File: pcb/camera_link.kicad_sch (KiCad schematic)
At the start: 12 parts, among them J1 RJ45_pyControl, J2 Screw_Terminal_01x08

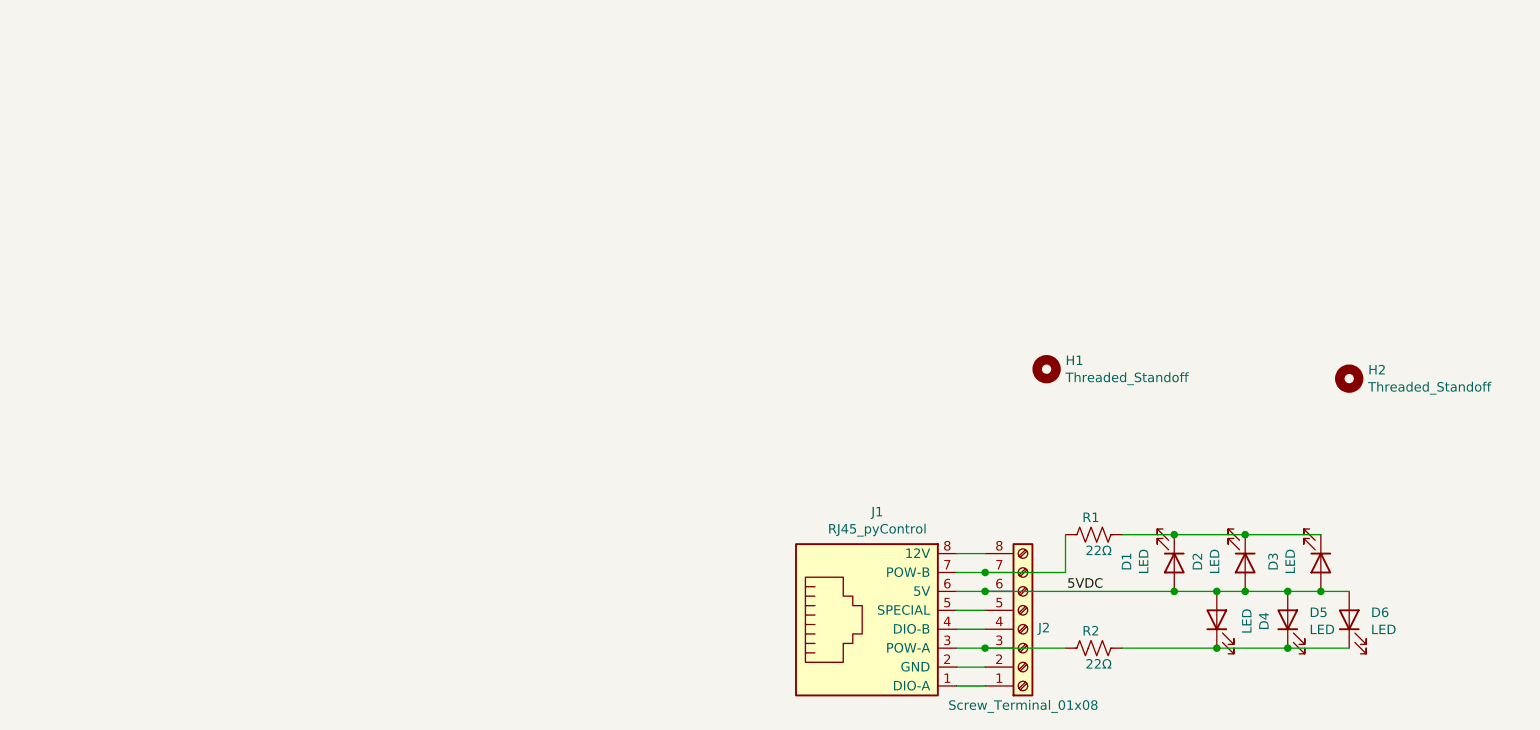
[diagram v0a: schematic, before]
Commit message: pcbv1.2
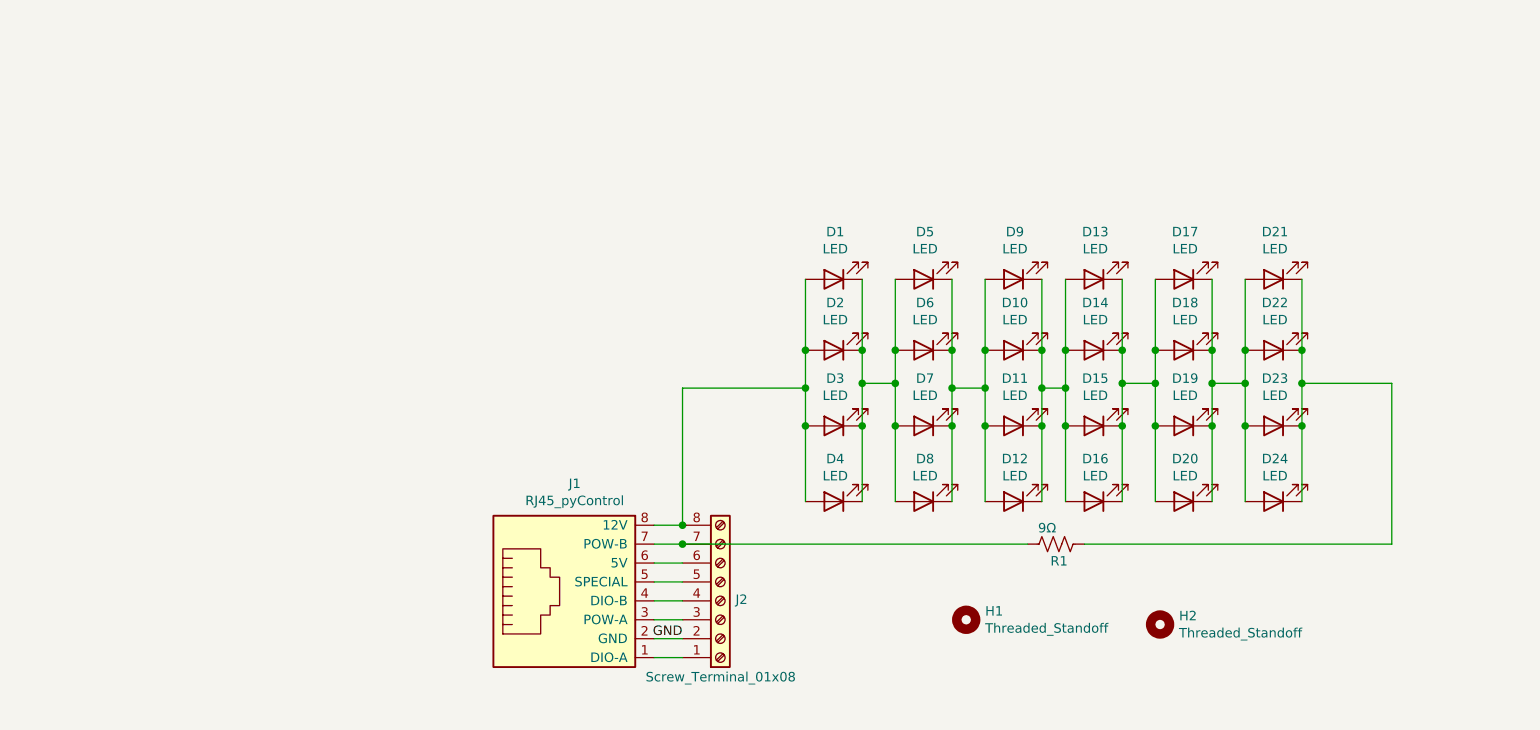
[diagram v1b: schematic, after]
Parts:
- removed R2: 22Ω, Resistor_THT:R_Axial_DIN0204_L3.6mm_D1.6mm_P7.62mm_Horizontal, symbol Device:R_US
- added D10, D11, D12, D13, D14, D15, D16, D17, D18, D19, D20, D21, D22, D23, D24, D7, D8, D9: LED, LED_SMD:LED_1206_3216Metric, symbol Device:LED
- J1: footprint asl_footprints:RJ45_THP_Vertical -> asl_footprints:RJ45_SMD
- R1: value 22Ω -> 9Ω; footprint Resistor_THT:R_Axial_DIN0204_L3.6mm_D1.6mm_P7.62mm_Horizontal -> Resistor_SMD:R_1206_3216Metric_Pad1.30x1.75mm_HandSolder
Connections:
- net GND: now reaches J1.2 (GND), J2.2 (Pin_2)
- net at J1.7 (POW-B), J2.7 (Pin_7): now also R1.2; no longer R1.1
- net at J1.8 (12V), J2.8 (Pin_8): now also D1.2 (A), D2.2 (A), D3.2 (A), D4.2 (A)
- net at D5.1 (K), D6.1 (K): now also D10.2 (A), D11.2 (A), D12.2 (A), D7.1 (K), D8.1 (K), D9.2 (A); no longer D4.1 (K)
- net at D1.1 (K), D2.1 (K), D3.1 (K): now also D4.1 (K), D5.2 (A), D6.2 (A), D7.2 (A), D8.2 (A); no longer R1.2
- removed net 5VDC: D1.2 (A), D2.2 (A), D3.2 (A), D4.2 (A), D5.2 (A), D6.2 (A), J1.6 (5V), J2.6 (Pin_6)
- new net: D17.1 (K), D18.1 (K), D19.1 (K), D20.1 (K), D21.2 (A), D22.2 (A), D23.2 (A), D24.2 (A)
- new net: D13.1 (K), D14.1 (K), D15.1 (K), D16.1 (K), D17.2 (A), D18.2 (A), D19.2 (A), D20.2 (A)
- new net: D10.1 (K), D11.1 (K), D12.1 (K), D13.2 (A), D14.2 (A), D15.2 (A), D16.2 (A), D9.1 (K)
- new net: J1.6 (5V), J2.6 (Pin_6)
- new net: D21.1 (K), D22.1 (K), D23.1 (K), D24.1 (K), R1.1
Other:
- moved on the sheet: D1, D2, D3, H1, H2, J1, J2, R1

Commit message: pcb v1.3
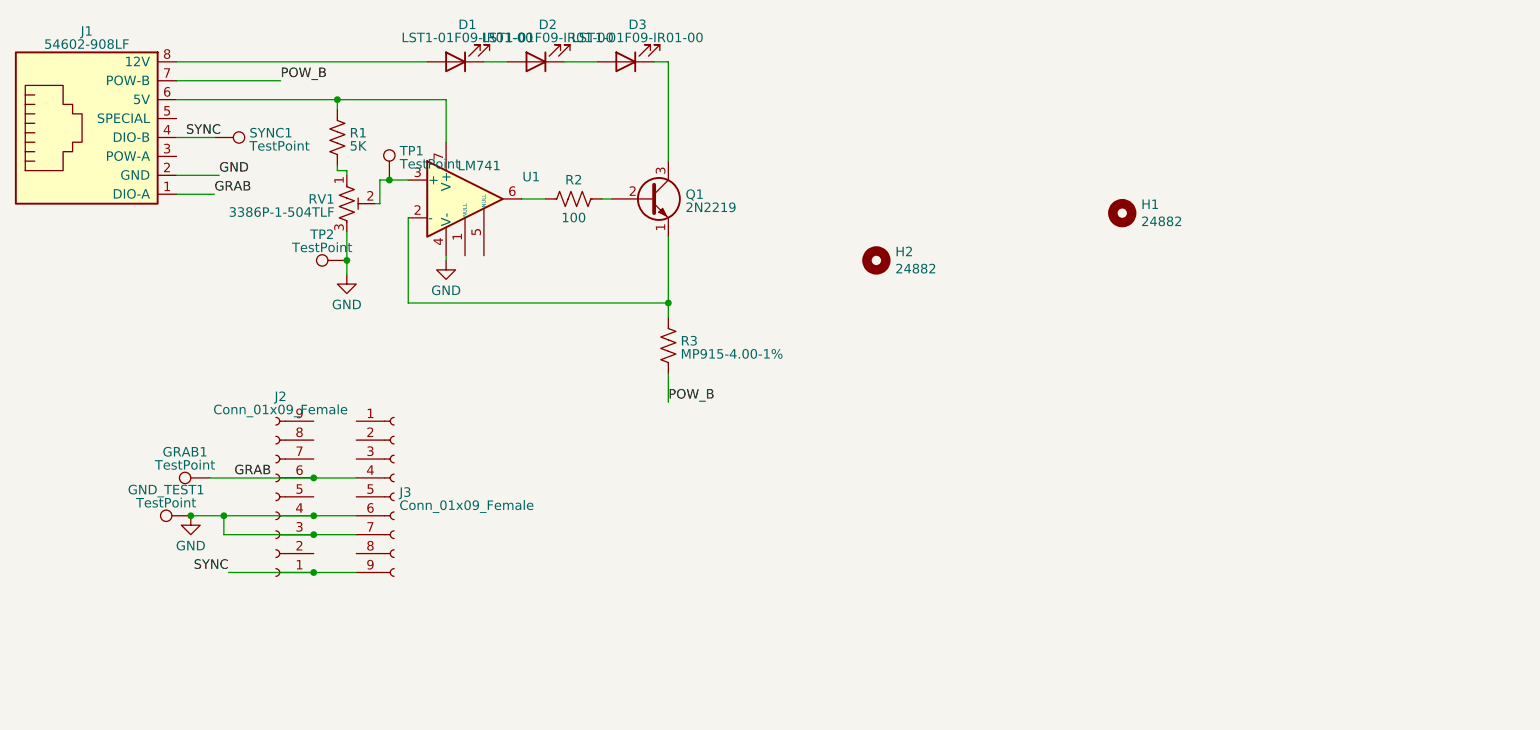
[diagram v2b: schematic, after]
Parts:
- removed D10, D11, D12, D13, D14, D15, D16, D17, D18, D19, D20, D21, D22, D23, D24, D4, D5, D6, D7, D8, D9: LED, LED_SMD:LED_1206_3216Metric, symbol Device:LED
- removed J2: Screw_Terminal_01x08, Connector_PinHeader_1.27mm:PinHeader_1x08_P1.27mm_Vertical, symbol Connector:Screw_Terminal_01x08
- added GND_TEST1, GRAB1, SYNC1, TP1, TP2: TestPoint, Connector_Pin:Pin_D1.0mm_L10.0mm, symbol Connector:TestPoint
- added J2, J3: Conn_01x09_Female, asl_footprints:JST_NSH_1x09_VERTICAL, symbol Connector:Conn_01x09_Female
- added Q1: 2N2219, Package_TO_SOT_SMD:SOT-23-6, symbol asl_symbols_new:NPN_transistor_ZXTC2045E6TA
- added R2: 100, Resistor_SMD:R_0805_2012Metric, symbol Device:R_US
- added R3: MP915-4.00-1%, asl_footprints:Resistor_power_MP900, symbol Device:R_US
- added RV1: 3386P-1-504TLF, Potentiometer_THT:Potentiometer_Bourns_3386P_Vertical, symbol Device:R_Potentiometer_Trim_US
- added U1: LM741, Package_DIP:DIP-8_W7.62mm, symbol Amplifier_Operational:LM741
- D1, D2, D3: value LED -> LST1-01F09-IR01-00; footprint LED_SMD:LED_1206_3216Metric -> asl_footprints:LED_starboard
- H1: renamed from H2; value Threaded_Standoff -> 24882; Sim_Device (none) -> SPICE; Sim_Params (none) -> type=H model="24882"
- H2: renamed from H1; value Threaded_Standoff -> 24882; Sim_Device (none) -> SPICE; Sim_Params (none) -> type=H model="24882"
- J1: value RJ45_pyControl -> 54602-908LF; footprint asl_footprints:RJ45_SMD -> asl_footprints:RJ45_THP
- R1: value 9Ω -> 5K; footprint Resistor_SMD:R_1206_3216Metric_Pad1.30x1.75mm_HandSolder -> Resistor_SMD:R_0805_2012Metric
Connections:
- net GND: now also GND_TEST1.1, J2.3 (Pin_3), J2.4 (Pin_4), J3.6 (Pin_6), J3.7 (Pin_7), RV1.3, TP2.1, U1.4 (V-)
- net GRAB: now reaches J1.1 (DIO-A)
- net GRAB: now also GRAB1.1, J2.6 (Pin_6), J3.4 (Pin_4)
- net SYNC: now reaches J1.4 (DIO-B)
- net SYNC: now also J2.1 (Pin_1), J3.9 (Pin_9), SYNC1.1
- net at J1.6 (5V): now also R1.1, U1.7 (V+)
- net at R1.2: now also RV1.1; no longer J1.7 (POW-B)
- net at D1.2 (A), J1.8 (12V): no longer D2.2 (A), D3.2 (A)
- new net: D2.1 (K), D3.2 (A)
- new net: D1.1 (K), D2.2 (A)
- new net: D3.1 (K), Q1.3 (C)
- new net: Q1.1 (E), R3.2, U1.2 (-)
- new net: RV1.2, TP1.1, U1.3 (+)
- new net: Q1.2 (B), R2.2
- new net: R2.1, U1.6
- new net POW_B: J1.7 (POW-B), R3.1
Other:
- moved on the sheet: H1, H2

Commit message: pcb v1.5
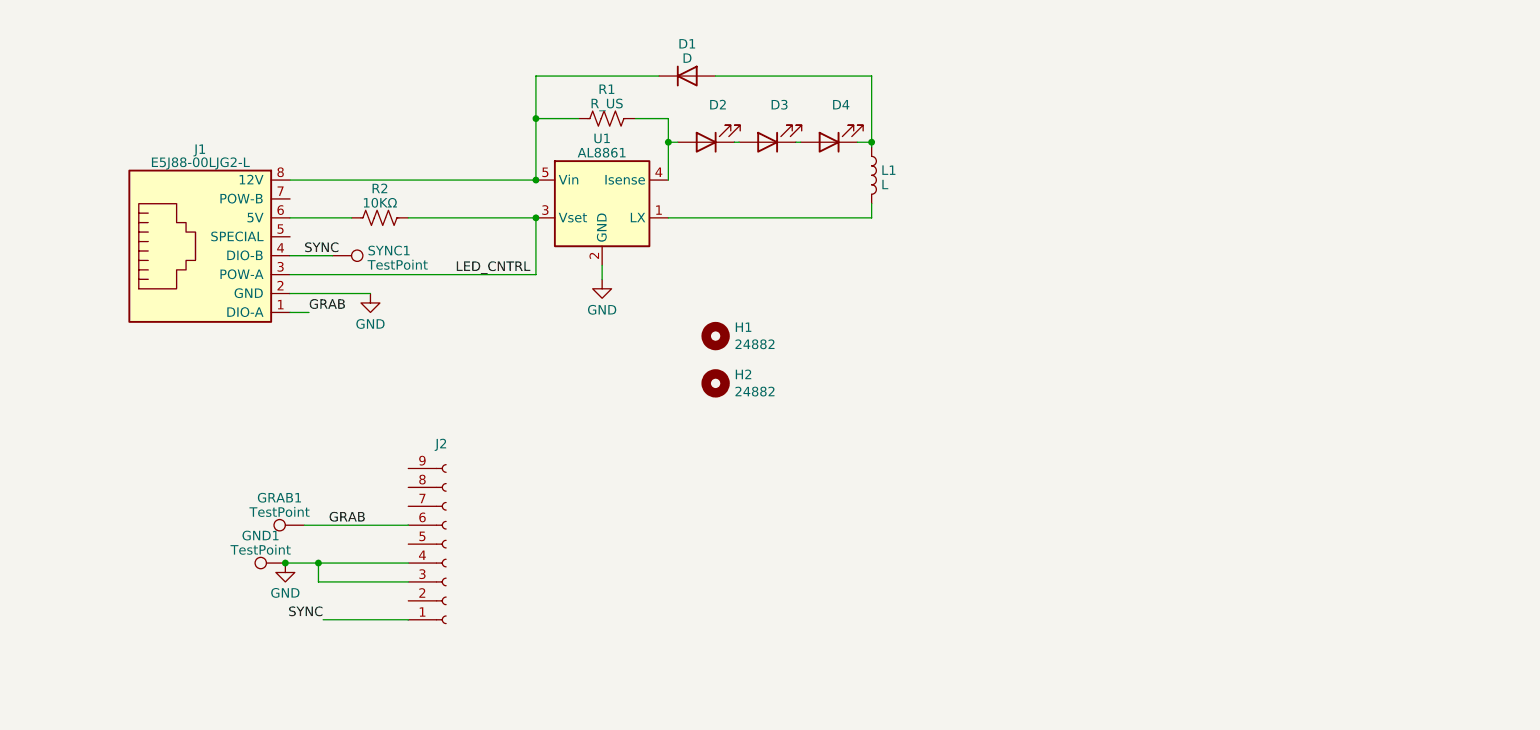
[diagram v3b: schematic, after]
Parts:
- removed D1: LST1-01F09-IR01-00, asl_footprints:LED_starboard, symbol Device:LED
- removed J3: Conn_01x09_Female, asl_footprints:JST_NSH_1x09_VERTICAL, symbol Connector:Conn_01x09_Female
- removed Q1: 2N2219, Package_TO_SOT_SMD:SOT-23-6, symbol asl_symbols_new:NPN_transistor_ZXTC2045E6TA
- removed R3: MP915-4.00-1%, asl_footprints:Resistor_power_MP900, symbol Device:R_US
- removed RV1: 3386P-1-504TLF, Potentiometer_THT:Potentiometer_Bourns_3386P_Vertical, symbol Device:R_Potentiometer_Trim_US
- removed TP1, TP2: TestPoint, Connector_Pin:Pin_D1.0mm_L10.0mm, symbol Connector:TestPoint
- removed U1: LM741, Package_DIP:DIP-8_W7.62mm, symbol Amplifier_Operational:LM741
- added D1: D, Diode_SMD:D_SMB, symbol Device:D
- added D4: LST1-01F09-IR01-00, asl_footprints:LED_starboard, symbol Device:LED
- added L1: L, Inductor_THT:L_Axial_L14.5mm_D5.8mm_P7.62mm_Vertical_Fastron_HBCC, symbol Device:L
- added U1: AL8861, Package_TO_SOT_SMD:SOT-89-5, symbol asl_symbols_new:AL8861
- H1: renamed from H2; Sim_Device SPICE -> (none); Sim_Params type=H model="24882" -> (none)
- H2: renamed from H1; Sim_Device SPICE -> (none); Sim_Params type=H model="24882" -> (none)
- J1: value 54602-908LF -> E5J88-00LJG2-L; footprint asl_footprints:RJ45_THP -> asl_footprints:RJ45_THP_tab_on_top
- R1: value 5K -> R_US; footprint Resistor_SMD:R_0805_2012Metric -> Resistor_THT:R_Axial_DIN0614_L14.3mm_D5.7mm_P7.62mm_Vertical
- R2: value 100 -> 10KΩ
- renumbered GND_TEST1 to GND1
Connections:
- net GND: now also U1.2 (GND)
- net at D2.2 (A): now also R1.2, U1.4 (Isense)
- net at J1.8 (12V): now also R1.1, D1.1 (K), U1.5 (Vin)
- net at J1.6 (5V): now also R2.1; no longer R1.1
- net at D3.1 (K): now also D4.2 (A)
- net LED_CNTRL: now reaches R2.2
- net LED_CNTRL: now also J1.3 (POW-A), U1.3 (Vset)
- net POW_B: no longer names the net of J1.7 (POW-B)
- new net: L1.2, U1.1 (LX)
- new net: D1.2 (A), D4.1 (K), L1.1
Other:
- moved on the sheet: GND1, GRAB1, H1, H2, J1, J2
